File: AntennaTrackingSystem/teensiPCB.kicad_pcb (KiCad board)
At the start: 2 copper layers, 45 x 84 mm, 12 parts, among them J1 screw terminal, J5 UART1, J6 UART2, J7 I2C ext, SW1 SW_Push, U1 Teensy4.1, U2 SAM-M10Q-00B

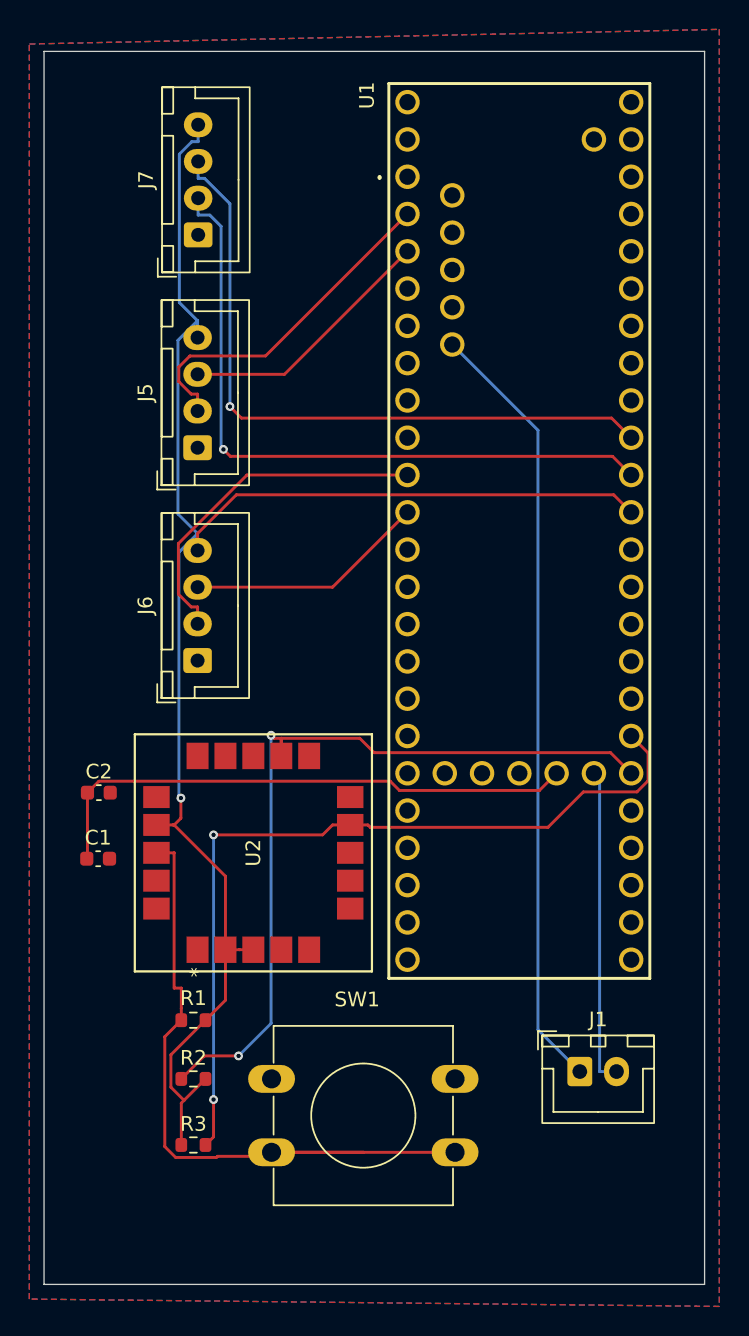
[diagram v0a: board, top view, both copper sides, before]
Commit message: forgot tracks
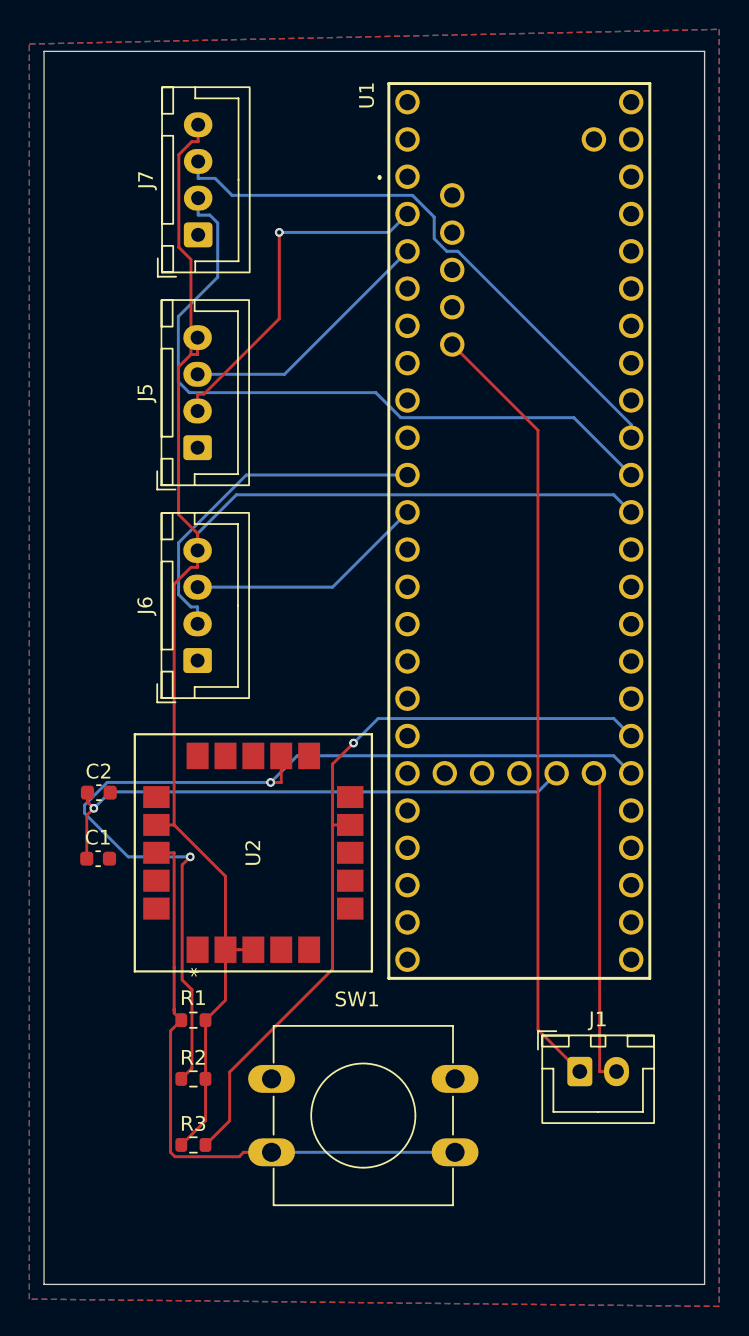
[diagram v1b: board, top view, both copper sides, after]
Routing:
- net Net-(U1-SCL): track 55.3 -> 66.6 mm
- net Net-(U2-RESET_N): track 48.6 -> 41.7 mm
- net Net-(J7-Pin_3): track 46.1 -> 39.4 mm, vias 1 -> 0
- net +3V3: track 115.9 -> 112.1 mm, vias 1 -> 0
- net Net-(U1-SDA): track 56.1 -> 52.9 mm, vias 2 -> 1
- net Net-(J7-Pin_2): track 46.8 -> 48.1 mm, vias 1 -> 0
- net Net-(J5-Pin_2): track 23.7 -> 24.0 mm, vias 0 -> 1
- net Net-(C1-Pad1): track 37.5 -> 37.4 mm, vias 0 -> 1
